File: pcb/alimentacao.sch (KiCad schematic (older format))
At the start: 5 parts, among them U3 LM317_SOT223

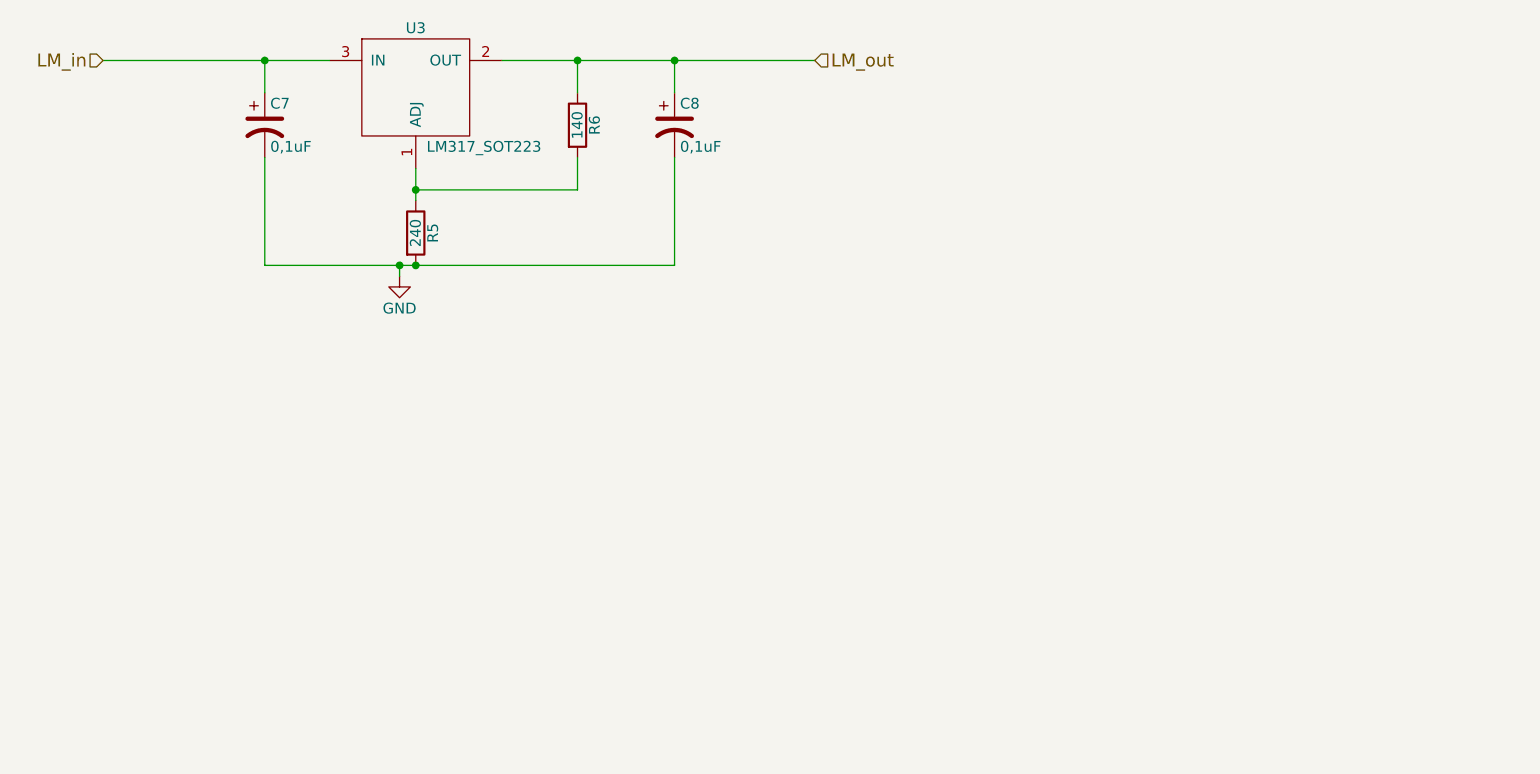
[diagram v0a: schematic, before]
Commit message: Clean up Kicad and TCC
Some changes in the
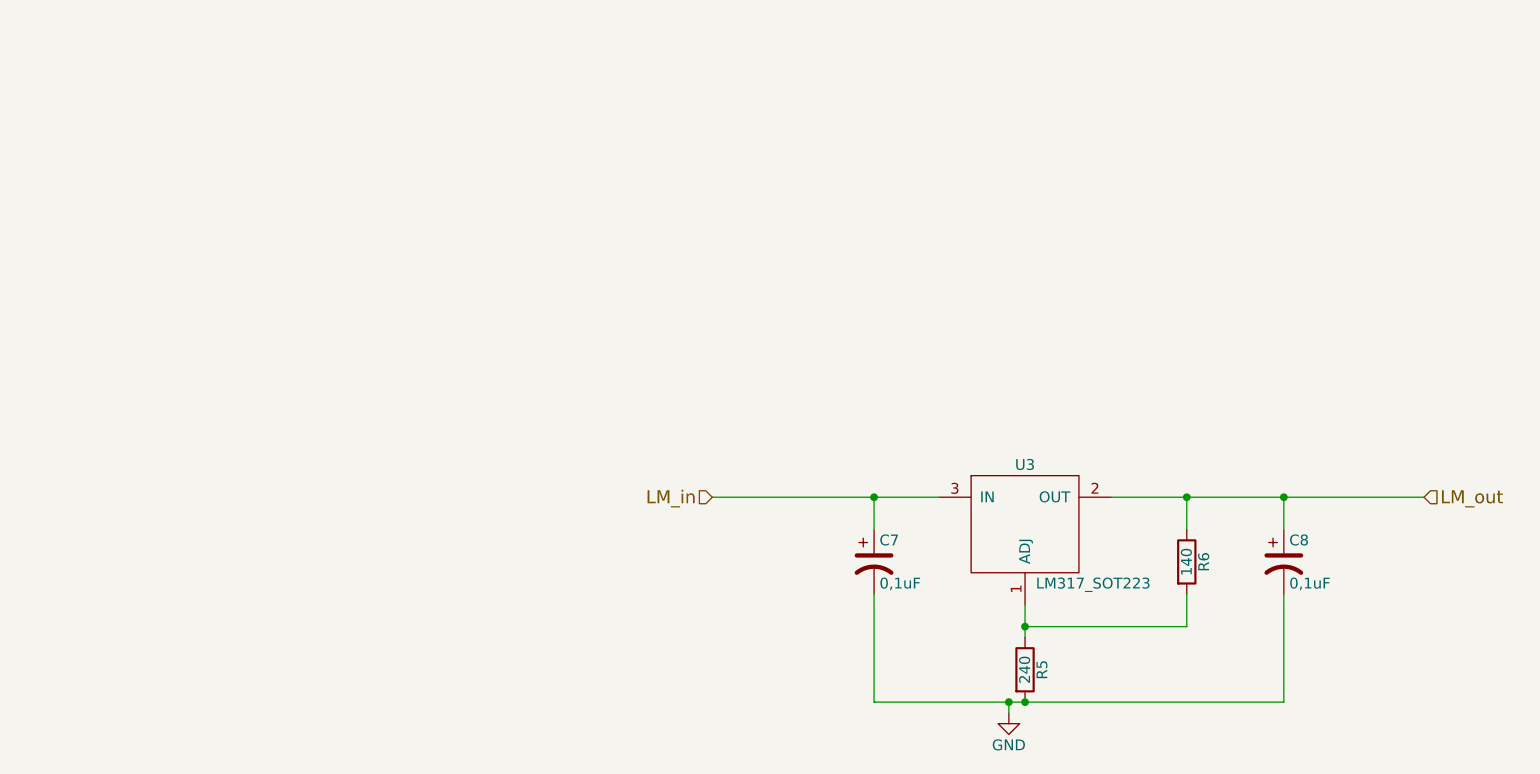
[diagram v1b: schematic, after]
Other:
- moved on the sheet: C7, C8, R5, R6, U3
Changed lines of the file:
@@
 encoding utf-8
 Sheet 2 10
-Title ""
+Title "Supply Schematic"
 Date ""
-Rev ""
-Comp ""
+Rev "1"
+Comp "Universidade de Brasília - Campus Gama"
 Comment1 ""
 Comment2 ""
@@
 L regul:LM317_SOT223 U3
 U 1 1 5AFC2FD4
-P 2800 1550
-F 0 "U3" H 2800 1850 50  0000 C CNN
-F 1 "LM317_SOT223" H 2850 1300 50  0000 L CNN
-F 2 "TO_SOT_Packages_SMD:SOT-223-3_TabPin2" H 2800 1550 50  0001 C CNN
-F 3 "https://www.digikey.com/product-detail/en/texas-instruments/LM317DCYR/296-12602-1-ND/443738" H 2800 1550 50  0001 C CNN
-	1    2800 1550
+P 5625 3575
+F 0 "U3" H 5625 3875 50  0000 C CNN
+F 1 "LM317_SOT223" H 5675 3325 50  0000 L CNN
+F 2 "TO_SOT_Packages_SMD:SOT-223-3_TabPin2" H 5625 3575 50  0001 C CNN
+F 3 "https://www.digikey.com/product-detail/en/texas-instruments/LM317DCYR/296-12602-1-ND/443738" H 5625 3575 50  0001 C CNN
+	1    5625 3575
 	1    0    0    -1
 $EndComp
@@
 L Device:R R5
 U 1 1 5AFC30F1
-P 2800 2200
-F 0 "R5" V 2880 2200 50  0000 C CNN
-F 1 "240" V 2800 2200 50  0000 C CNN
-F 2 "Resistors_SMD:R_1206" V 2730 2200 50  0001 C CNN
-F 3 "https://www.digikey.com/product-detail/en/panasonic-electronic-components/ERA-8AEB241V/P240BCCT-ND/3069680" H 2800 2200 50  0001 C CNN
-	1    2800 2200
+P 5625 4225
+F 0 "R5" V 5705 4225 50  0000 C CNN
+F 1 "240" V 5625 4225 50  0000 C CNN
+F 2 "Resistors_SMD:R_1206" V 5555 4225 50  0001 C CNN
+F 3 "https://www.digikey.com/product-detail/en/panasonic-electronic-components/ERA-8AEB241V/P240BCCT-ND/3069680" H 5625 4225 50  0001 C CNN
+	1    5625 4225
 	1    0    0    -1
 $EndComp
@@
 L Device:R R6
 U 1 1 5AFC3148
-P 3550 1700
-F 0 "R6" V 3630 1700 50  0000 C CNN
-F 1 "140" V 3550 1700 50  0000 C CNN
-F 2 "Resistors_SMD:R_1206" V 3480 1700 50  0001 C CNN
-F 3 "https://www.digikey.com/product-detail/en/stackpole-electronics-inc/RMCF1206FT140R/RMCF1206FT140RCT-ND/2418574" H 3550 1700 50  0001 C CNN
-	1    3550 1700
+P 6375 3725
+F 0 "R6" V 6455 3725 50  0000 C CNN
+F 1 "140" V 6375 3725 50  0000 C CNN
+F 2 "Resistors_SMD:R_1206" V 6305 3725 50  0001 C CNN
+F 3 "https://www.digikey.com/product-detail/en/stackpole-electronics-inc/RMCF1206FT140R/RMCF1206FT140RCT-ND/2418574" H 6375 3725 50  0001 C CNN
+	1    6375 3725
 	1    0    0    -1
 $EndComp
@@
 L Device:CP1 C7
 U 1 1 5AFC316F
-P 2100 1700
-F 0 "C7" H 2125 1800 50  0000 L CNN
-F 1 "0,1uF" H 2125 1600 50  0000 L CNN
-F 2 "Capacitors_SMD:C_1206" H 2100 1700 50  0001 C CNN
-F 3 "https://www.digikey.com/product-detail/en/avx-corporation/TAJA104K035RNJ/478-2368-2-ND/678452" H 2100 1700 50  0001 C CNN
-	1    2100 1700
+P 4925 3725
+F 0 "C7" H 4950 3825 50  0000 L CNN
+F 1 "0,1uF" H 4950 3625 50  0000 L CNN
+F 2 "Capacitors_SMD:C_1206" H 4925 3725 50  0001 C CNN
+F 3 "https://www.digikey.com/product-detail/en/avx-corporation/TAJA104K035RNJ/478-2368-2-ND/678452" H 4925 3725 50  0001 C CNN
+	1    4925 3725
 	1    0    0    -1
 $EndComp
@@
 L Device:CP1 C8
 U 1 1 5AFC318C
-P 4000 1700
-F 0 "C8" H 4025 1800 50  0000 L CNN
-F 1 "0,1uF" H 4025 1600 50  0000 L CNN
-F 2 "Capacitors_SMD:C_1206" H 4000 1700 50  0001 C CNN
-F 3 "https://www.digikey.com/product-detail/en/avx-corporation/TAJA104K035RNJ/478-2368-2-ND/678452" H 4000 1700 50  0001 C CNN
-	1    4000 1700
+P 6825 3725
+F 0 "C8" H 6850 3825 50  0000 L CNN
+F 1 "0,1uF" H 6850 3625 50  0000 L CNN
+F 2 "Capacitors_SMD:C_1206" H 6825 3725 50  0001 C CNN
+F 3 "https://www.digikey.com/product-detail/en/avx-corporation/TAJA104K035RNJ/478-2368-2-ND/678452" H 6825 3725 50  0001 C CNN
+	1    6825 3725
 	1    0    0    -1
 $EndComp
 Wire Wire Line
-	1350 1400 2100 1400
+	4175 3425 4925 3425
 Wire Wire Line
-	2100 1400 2100 1550
+	4925 3425 4925 3575
 Wire Wire Line
-	2800 1900 2800 2000
+	5625 3925 5625 4025
 Wire Wire Line
-	2100 2350 2725 2350
+	4925 4375 5550 4375
 Wire Wire Line
-	2100 2350 2100 1850
+	4925 4375 4925 3875
 Wire Wire Line
-	3200 1400 3550 1400
+	6025 3425 6375 3425
 Wire Wire Line
-	3550 1400 3550 1550
+	6375 3425 6375 3575
 Wire Wire Line
-	3550 1850 3550 2000
+	6375 3875 6375 4025
 Wire Wire Line
-	3550 2000 2800 2000
-Connection ~ 2800 2000
+	6375 4025 5625 4025
+Connection ~ 5625 4025
 Wire Wire Line
-	4000 1400 4000 1550
-Connection ~ 3550 1400
+	6825 3425 6825 3575
+Connection ~ 6375 3425
 Wire Wire Line
-	4000 2350 4000 1850
-Connection ~ 2800 2350
+	6825 4375 6825 3875
+Connection ~ 5625 4375
 $Comp
 L power:GND #PWR04
 U 1 1 5AFC3327
-P 2725 2400
-F 0 "#PWR04" H 2725 2150 50  0001 C CNN
-F 1 "GND" H 2725 2250 50  0000 C CNN
-F 2 "" H 2725 2400 50  0001 C CNN
-F 3 "" H 2725 2400 50  0001 C CNN
-	1    2725 2400
+P 5550 4425
+F 0 "#PWR04" H 5550 4175 50  0001 C CNN
+F 1 "GND" H 5550 4275 50  0000 C CNN
+F 2 "" H 5550 4425 50  0001 C CNN
+F 3 "" H 5550 4425 50  0001 C CNN
+	1    5550 4425
 	1    0    0    -1
 $EndComp
-Connection ~ 2100 1400
-Connection ~ 4000 1400
-Text HLabel 1350 1400 0    60   Input ~ 0
+Connection ~ 4925 3425
+Connection ~ 6825 3425
+Text HLabel 4175 3425 0    60   Input ~ 0
 LM_in
-Text HLabel 4650 1400 2    60   Input ~ 0
+Text HLabel 7475 3425 2    60   Input ~ 0
 LM_out
 Wire Wire Line
-	2725 2400 2725 2350
-Connection ~ 2725 2350
+	5550 4425 5550 4375
+Connection ~ 5550 4375
 Wire Wire Line
-	2800 2000 2800 2050
+	5625 4025 5625 4075
 Wire Wire Line
-	3550 1400 4000 1400
+	6375 3425 6825 3425
 Wire Wire Line
-	2800 2350 4000 2350
+	5625 4375 6825 4375
 Wire Wire Line
-	2100 1400 2400 1400
+	4925 3425 5225 3425
 Wire Wire Line
-	4000 1400 4650 1400
+	6825 3425 7475 3425
 Wire Wire Line
-	2725 2350 2800 2350
+	5550 4375 5625 4375
 $EndSCHEMATC
